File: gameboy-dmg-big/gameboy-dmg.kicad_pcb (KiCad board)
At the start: 2 copper layers, 82.5 x 139.7 mm, 95 parts, among them J1 Conn_01x02, J2 USB_A, J3 Conn_01x08, J4 Conn_01x04, J5 Raspberry_Pi_2_3, J7 USB_B_Micro, J8 Conn_01x02, P1 RK10J_POT, Q1 S8050, SW1 SW_DPDT_x2, U1 MCP23017_SO, U2 TP4056, U3 FS312F-G, U4 FS8205, U5 MT3608, U6 PAM8302AAS, U7 XC6206PxxxMR

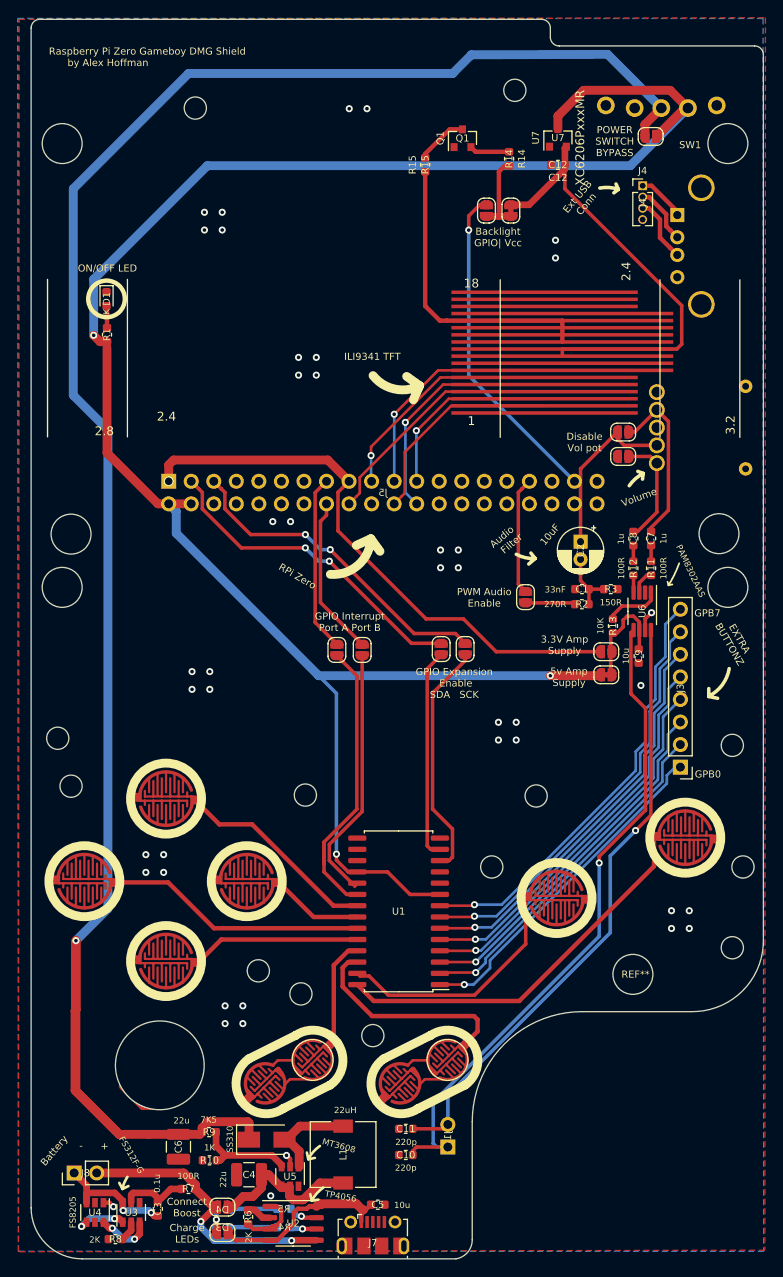
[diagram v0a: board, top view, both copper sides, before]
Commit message: Little board gerbers
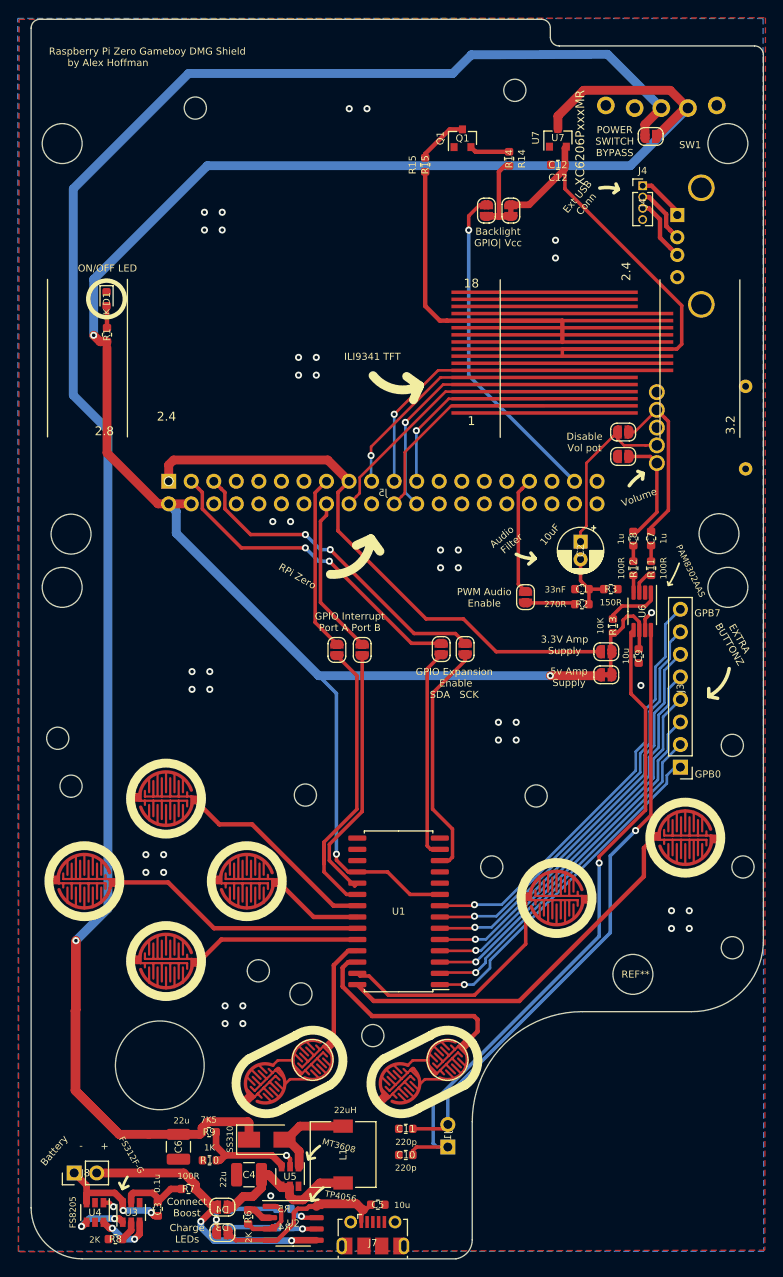
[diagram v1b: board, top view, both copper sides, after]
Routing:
- net (no net): track 5.85 -> 0.75 mm
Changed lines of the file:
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@@
     (thickness 1.6)
     (drawings 77)
-    (tracks 587)
+    (tracks 590)
     (zones 0)
     (modules 95)
@@
   )
   (setup
-    (last_trace_width 0.3)
+    (last_trace_width 0.5)
     (user_trace_width 0.3)
     (user_trace_width 0.4)
@@
     (add_net "Net-(U6-Pad2)")
   )
+  (module MountingHole:MountingHole_2.5mm (layer F.Cu)
+    (at 93.5 130.95)
+    (descr "Mounting Hole 2.5mm, no annular")
+    (tags "mounting hole 2.5mm no annular")
+    (attr virtual)
+    (fp_text reference REF** (at 0 -3.5) (layer F.SilkS) hide
+      (effects (font (size 0.8 0.8) (thickness 0.15)))
+    )
+    (fp_text value MountingHole_2.5mm (at 0 3.5) (layer F.SilkS) hide
+      (effects (font (size 0.7 0.7) (thickness 0.12)))
+    )
+    (fp_text user %R (at 0.3 0) (layer F.SilkS) hide
+      (effects (font (size 0.8 0.8) (thickness 0.15)))
+    )
+    (fp_circle (center 0 0) (end 2.5 0) (layer Cmts.User) (width 0.15))
+    (fp_circle (center 0 0) (end 2.75 0) (layer F.CrtYd) (width 0.05))
+    (pad "" np_thru_hole circle (at 0 0) (size 10 10) (drill 10) (layers *.Cu *.Mask))
+  )
   (module pad:Tux (layer B.Cu)
     (at 102.6 100.85 200)
@@
     )
   )
-  (module MountingHole:MountingHole_2.5mm (layer F.Cu)
-    (at 93.5 130.95)
-    (descr "Mounting Hole 2.5mm, no annular")
-    (tags "mounting hole 2.5mm no annular")
-    (attr virtual)
-    (fp_text reference REF** (at 0 -3.5) (layer F.SilkS) hide
-      (effects (font (size 0.8 0.8) (thickness 0.15)))
-    )
-    (fp_text value MountingHole_2.5mm (at 0 3.5) (layer F.SilkS) hide
-      (effects (font (size 0.7 0.7) (thickness 0.12)))
-    )
-    (fp_text user %R (at 0.3 0) (layer F.SilkS) hide
-      (effects (font (size 0.8 0.8) (thickness 0.15)))
-    )
-    (fp_circle (center 0 0) (end 2.5 0) (layer Cmts.User) (width 0.15))
-    (fp_circle (center 0 0) (end 2.75 0) (layer F.CrtYd) (width 0.05))
-    (pad "" np_thru_hole circle (at 0 0) (size 10 10) (drill 10) (layers *.Cu *.Mask))
-  )
   (module Connector_PinHeader_2.54mm:PinHeader_2x20_P2.54mm_Vertical (layer B.Cu)
     (at 94.5 65.15 270)
@@
   (gr_line (start 161.5 17.080241) (end 161.5 116.8) (layer Edge.Cuts) (width 0.05))
   (segment (start 135.65 101.2) (end 135.65 100.452408) (width 0.4) (layer F.Cu) (net 0))
-  (segment (start 93.4 135.6) (end 91.55 135.6) (width 0.75) (layer F.Cu) (net 0))
-  (segment (start 91.55 135.6) (end 89.25 133.3) (width 0.75) (layer F.Cu) (net 0))
   (segment (start 140.9 76.35) (end 141.85 77.3) (width 0.4) (layer F.Cu) (net 1))
   (segment (start 140.9 73.95) (end 140.9 76.35) (width 0.4) (layer F.Cu) (net 1))
@@
   (segment (start 117.59501 123.70001) (end 133.99999 123.70001) (width 0.5) (layer F.Cu) (net 6))
   (segment (start 115.75 121.855) (end 117.59501 123.70001) (width 0.5) (layer F.Cu) (net 6))
-  (segment (start 149.180935 105.881903) (end 149.110839 105.626049) (width 0.5) (layer F.Cu) (net 6))
-  (segment (start 133.99999 123.70001) (end 149.180935 108.519065) (width 0.5) (layer F.Cu) (net 6))
-  (segment (start 149.180935 108.519065) (end 149.180935 105.881903) (width 0.5) (layer F.Cu) (net 6))
+  (segment (start 149.04 105.47) (end 149.046001 105.144217) (width 0.5) (layer F.Cu) (net 6))
+  (segment (start 148.0375 106.4725) (end 149.04 105.47) (width 0.5) (layer F.Cu) (net 6))
+  (segment (start 148.0375 109.6625) (end 148.0375 106.4725) (width 0.5) (layer F.Cu) (net 6))
+  (segment (start 133.99999 123.70001) (end 148.0375 109.6625) (width 0.5) (layer F.Cu) (net 6))
   (segment (start 117.085 120.885) (end 119.25 123.05) (width 0.4) (layer F.Cu) (net 7))
   (segment (start 115.75 120.585) (end 116.05 120.885) (width 0.4) (layer F.Cu) (net 7))
@@
   (segment (start 140.1125 78.85) (end 140.2625 79) (width 0.4) (layer F.Cu) (net 80))
   (segment (start 134.7 78.85) (end 140.1125 78.85) (width 0.4) (layer F.Cu) (net 80))
-  (segment (start 147 59.6) (end 149.5 57.1) (width 0.4) (layer F.Cu) (net 81))
-  (segment (start 146.35 59.6) (end 147 59.6) (width 0.4) (layer F.Cu) (net 81))
   (segment (start 150.399999 57.999999) (end 149.5 57.1) (width 0.4) (layer F.Cu) (net 81))
   (segment (start 150.800001 58.400001) (end 150.399999 57.999999) (width 0.4) (layer F.Cu) (net 81))
@@
   (segment (start 148.85 70.3625) (end 150.800001 68.412499) (width 0.4) (layer F.Cu) (net 81))
   (segment (start 148.85 70.8) (end 148.85 70.3625) (width 0.4) (layer F.Cu) (net 81))
+  (segment (start 147 59.6) (end 149.5 57.1) (width 0.3) (layer F.Cu) (net 81))
+  (segment (start 146.35 59.6) (end 147 59.6) (width 0.3) (layer F.Cu) (net 81))
   (segment (start 148.85 72.375) (end 148.85 74.1625) (width 0.4) (layer F.Cu) (net 82))
   (segment (start 146.85 72.3875) (end 146.85 74.1625) (width 0.4) (layer F.Cu) (net 83))
@@
   (segment (start 145.575 79.2) (end 148.217478 79.2) (width 0.4) (layer F.Cu) (net 89))
   (segment (start 148.217478 79.2) (end 148.825 78.592478) (width 0.4) (layer F.Cu) (net 89))
-  (segment (start 145.05 60.347592) (end 145.05 59.6) (width 0.4) (layer F.Cu) (net 91))
-  (segment (start 145.802408 61.1) (end 145.05 60.347592) (width 0.4) (layer F.Cu) (net 91))
-  (segment (start 149.5 61.1) (end 145.802408 61.1) (width 0.4) (layer F.Cu) (net 91))
-  (segment (start 140.9 63.75) (end 145.05 59.6) (width 0.4) (layer F.Cu) (net 91))
-  (segment (start 140.9 71.95) (end 140.9 63.75) (width 0.4) (layer F.Cu) (net 91))
+  (segment (start 141.559999 63.090001) (end 144.595936 60.054064) (width 0.3) (layer F.Cu) (net 91))
+  (segment (start 141.559999 70.190001) (end 141.559999 63.090001) (width 0.3) (layer F.Cu) (net 91))
+  (segment (start 140.9 70.85) (end 141.559999 70.190001) (width 0.3) (layer F.Cu) (net 91))
+  (segment (start 144.595936 60.054064) (end 145.05 59.6) (width 0.3) (layer F.Cu) (net 91))
+  (segment (start 140.9 71.95) (end 140.9 70.85) (width 0.3) (layer F.Cu) (net 91))
+  (segment (start 145.802408 61.1) (end 148.227208 61.1) (width 0.3) (layer F.Cu) (net 91))
+  (segment (start 145.05 60.347592) (end 145.802408 61.1) (width 0.3) (layer F.Cu) (net 91))
+  (segment (start 148.227208 61.1) (end 149.5 61.1) (width 0.3) (layer F.Cu) (net 91))
+  (segment (start 145.05 59.6) (end 145.05 60.347592) (width 0.3) (layer F.Cu) (net 91))
   (segment (start 148.75 62.35) (end 149.5 63.1) (width 0.4) (layer F.Cu) (net 92))
   (segment (start 146.35 62.35) (end 148.75 62.35) (width 0.4) (layer F.Cu) (net 92))
